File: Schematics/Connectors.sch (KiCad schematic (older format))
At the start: 82 parts, among them P605 CONN_02X05, P607 CONN_02X05, P608 CONN_02X05, P609 CONN_02X20, P610 CONN_02X05, P611 CONN_02X05, P612 CONN_02X05

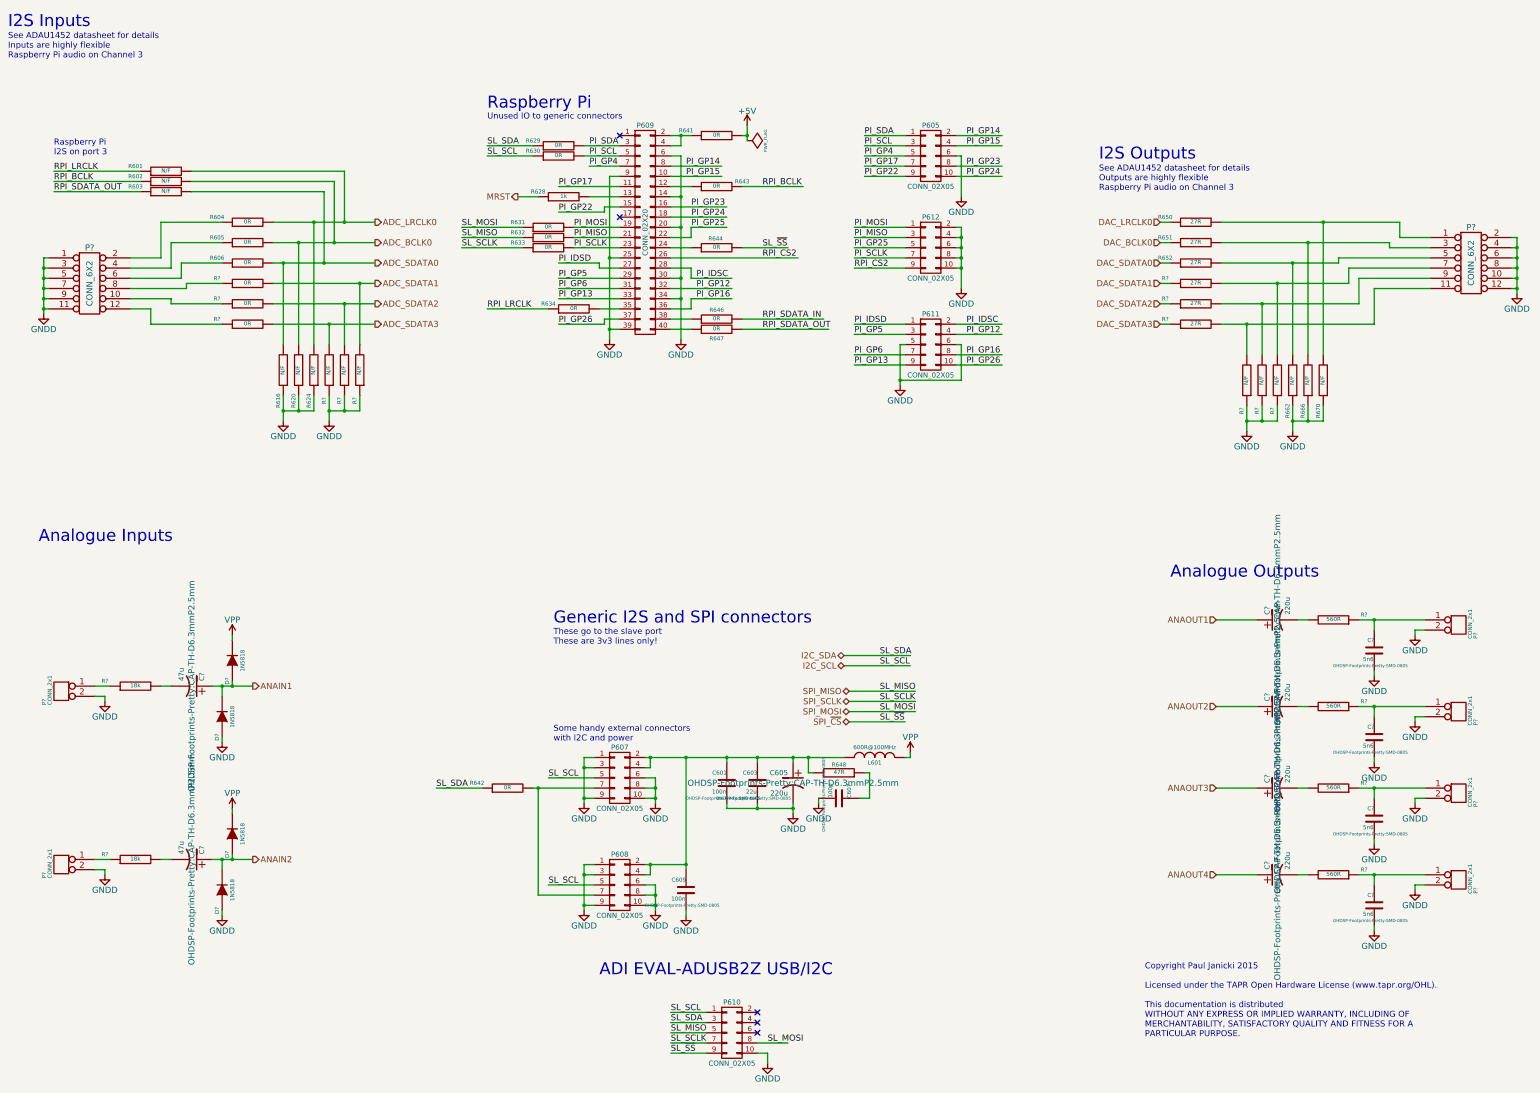
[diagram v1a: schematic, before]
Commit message: WIP
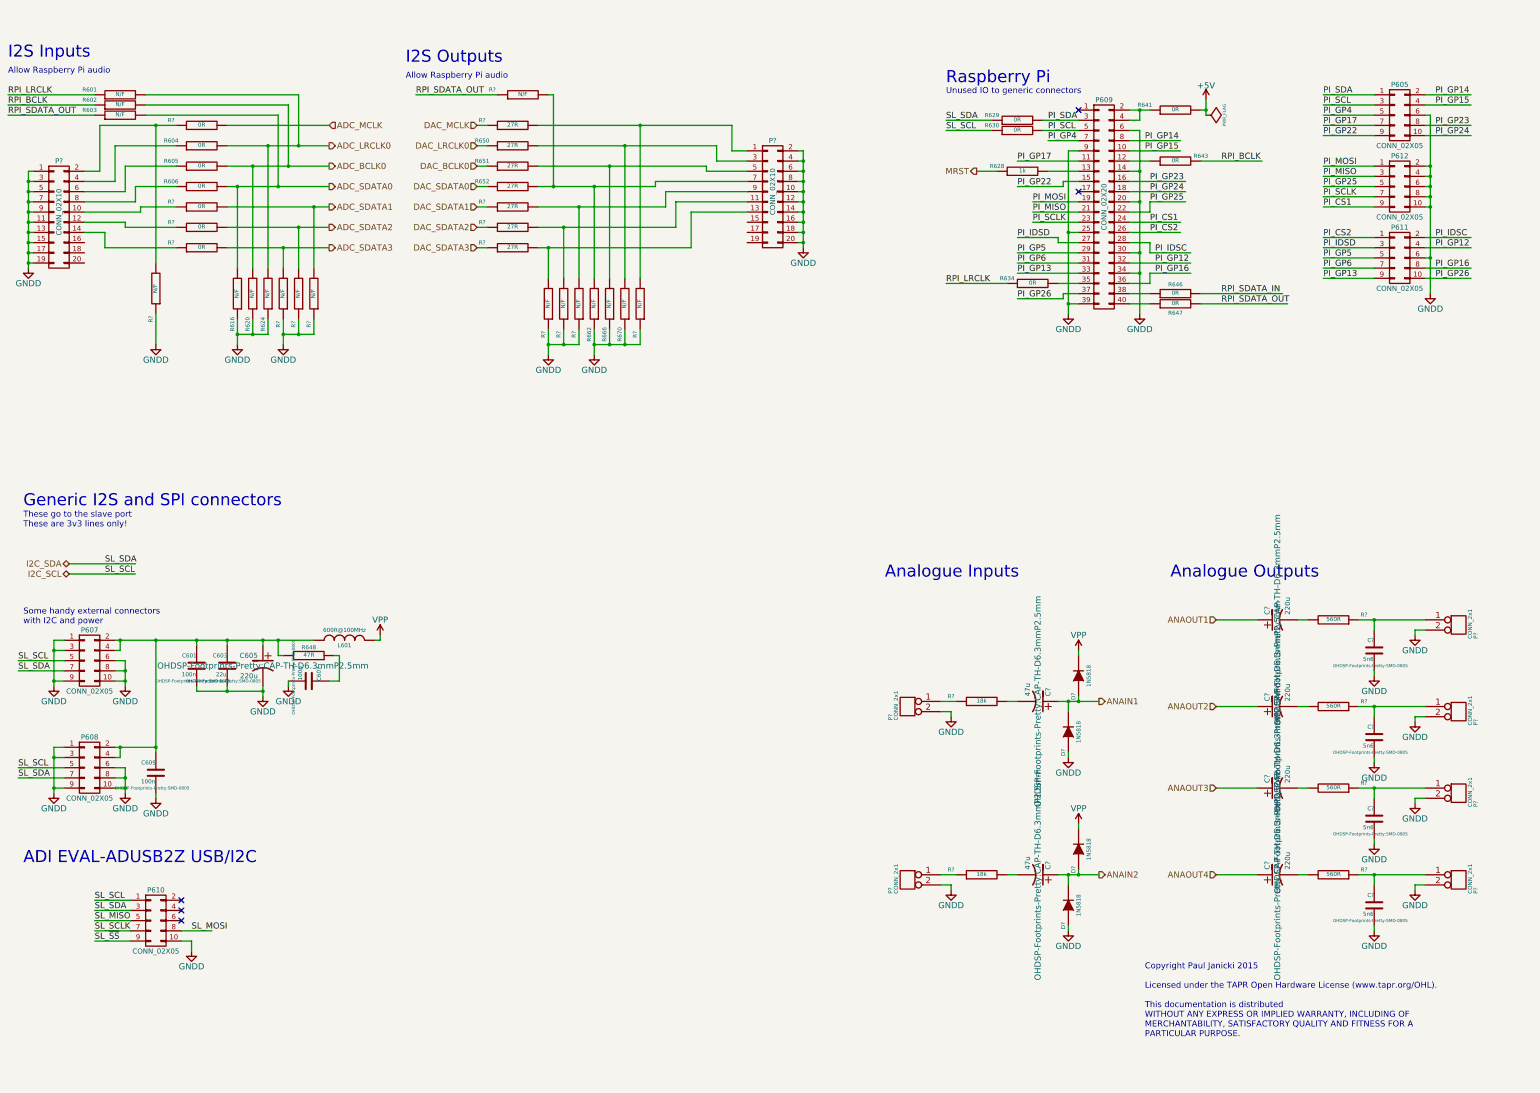
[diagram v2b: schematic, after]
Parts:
- removed P? (x2): CONN_6X2, symbol CONN_6X2
- removed R631, R632, R633, R642, R644: 0R, OHDSP-Footprints-Pretty:SMD-0805, symbol R
- added P? (x2): CONN_02X10, symbol CONN_02X10
- added R?: 0R, OHDSP-Footprints-Pretty:SMD-0603, symbol R
- added R? (x2): N/F, OHDSP-Footprints-Pretty:SMD-0603, symbol R
- added R?: 27R, OHDSP-Footprints-Pretty:SMD-0603, symbol R
- added R?: N/F, OHDSP-Footprints-Pretty:SMD-0805, symbol R
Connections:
- net labels added: ADC_MCLK, DAC_MCLK, PI_CS1, PI_CS2
- net labels removed: RPI_CS2, SPI_MISO, SPI_MOSI, SPI_SCLK, SPI_~CS
- wire segments 305 -> 314
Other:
- note added: "Allow Raspberry Pi audio"
- note removed: "Raspberry Pi\nI2S on port 3"
- note removed: "See ADAU1452 datasheet for details\nInputs are highly flexible\nRaspberry Pi audio on Channel 3"
- note removed: "See ADAU1452 datasheet for details\nOutputs are highly flexible\nRaspberry Pi audio on Channel 3"
- moved on the sheet: C601, C603, C605, C607, C609, C?, D?, L601, P605, P607, P608, P609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
